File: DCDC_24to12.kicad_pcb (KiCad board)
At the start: 2 copper layers, 69.8 x 29.8 mm, 28 parts, among them J1 Power_IN, J2 Power_OUT, U1 BD9F800MUX-ZE2

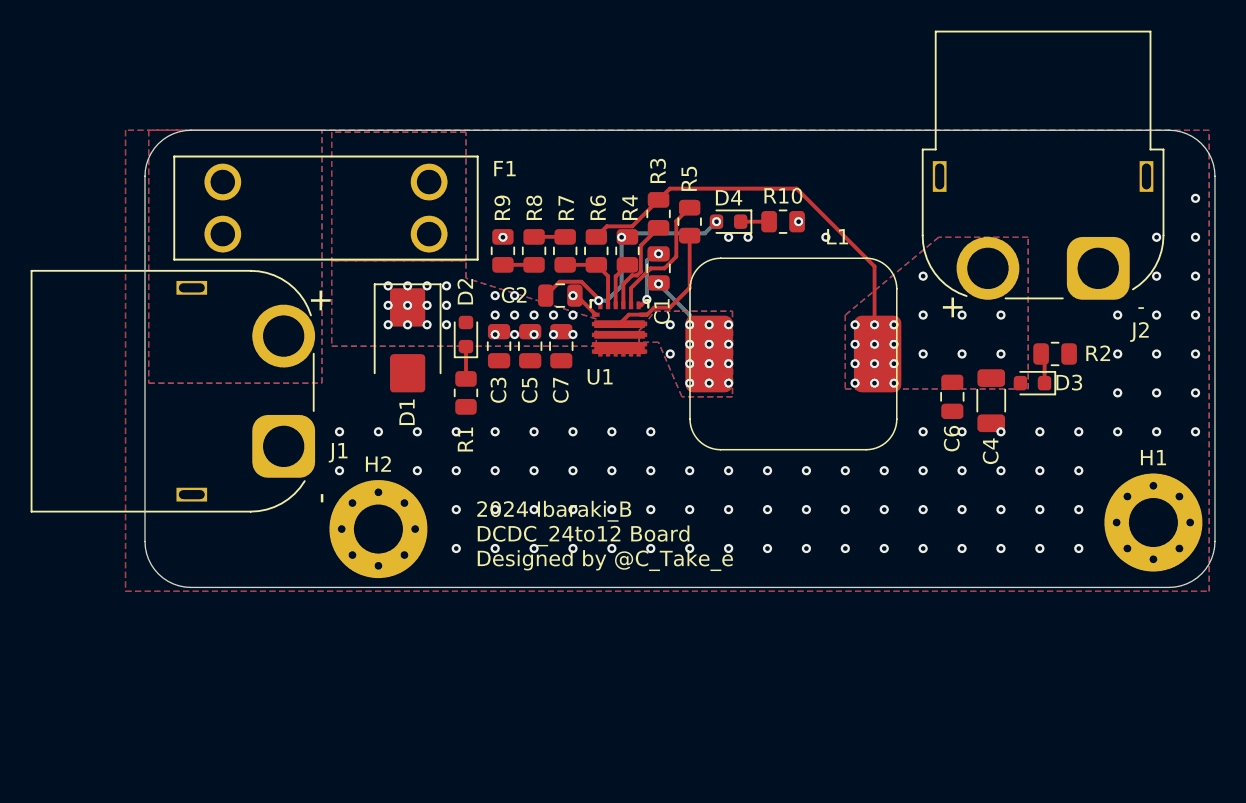
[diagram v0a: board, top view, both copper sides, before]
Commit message: 配置変更案 詳細未設定
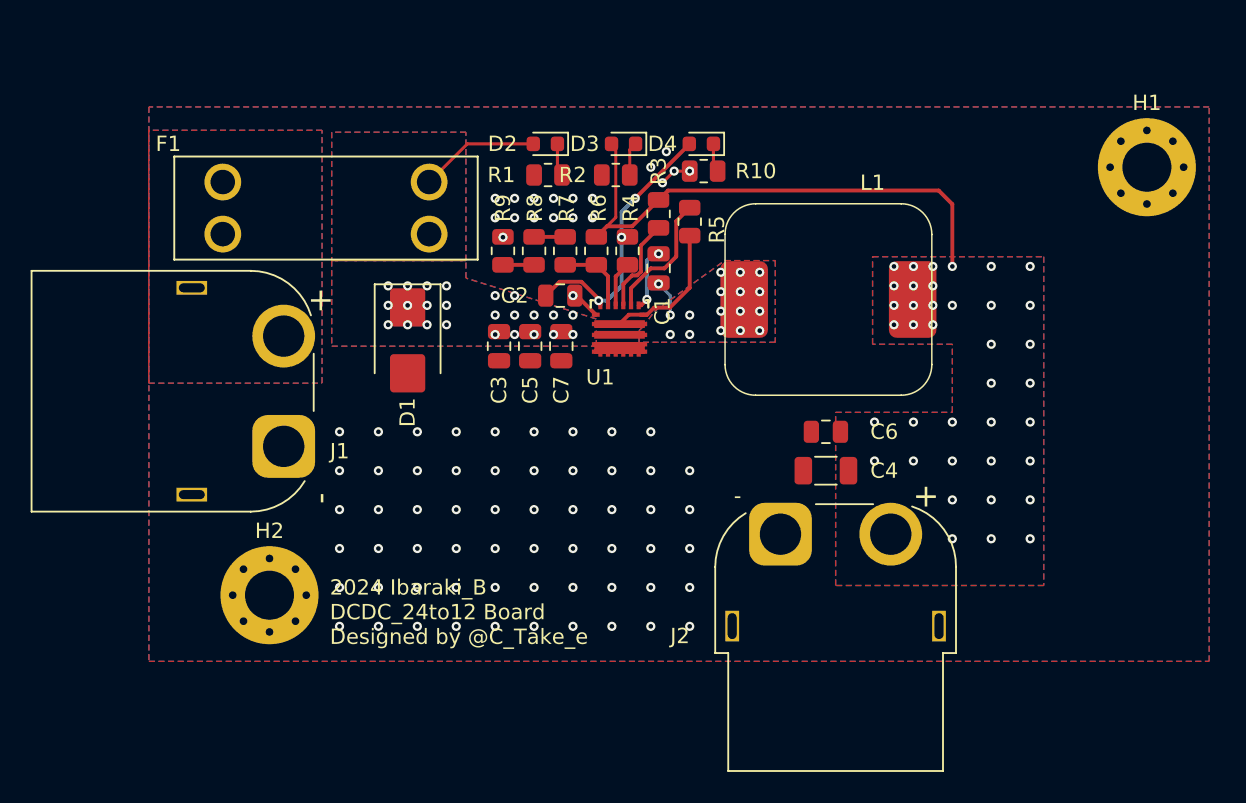
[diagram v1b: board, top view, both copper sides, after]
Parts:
- moved R2 31.0 mm to (101.9, 44.2), turned to 180 degrees
- moved D3 30.9 mm to (102.4, 42.2)
- moved J2 27.0 mm to (112.6, 67.6), turned to 180 degrees
- moved H1 23.2 mm to (136.5, 43.7)
- moved R1 15.2 mm to (97.4, 44.2), turned to 180 degrees
- moved D2 13.5 mm to (97.3, 42.2), turned to 180 degrees
- moved C4 11.7 mm to (115.6, 63.5), turned to 180 degrees
- moved C6 8.57 mm to (115.6, 61.0), turned to 180 degrees
- moved H2 8.32 mm to (79.2, 71.6)
- moved R10 6.15 mm to (107.6, 43.9), turned to 180 degrees
- moved D4 5.38 mm to (107.4, 42.2)
- moved L1 4.23 mm to (110.2, 52.3)
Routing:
- net +12V: track 25.4 -> 34.7 mm, vias 19 -> 38
- net +BATT: track 8.97 -> 16.8 mm
- net GND: track 2.73 -> 4.82 mm, vias 90 -> 78
- net VREG: track 16.4 -> 17.8 mm
- net SW: track 3.51 -> 2.35 mm, vias 15 -> 17
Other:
- board outline removed
